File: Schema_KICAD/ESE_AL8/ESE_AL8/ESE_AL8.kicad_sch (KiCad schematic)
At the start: 4 parts

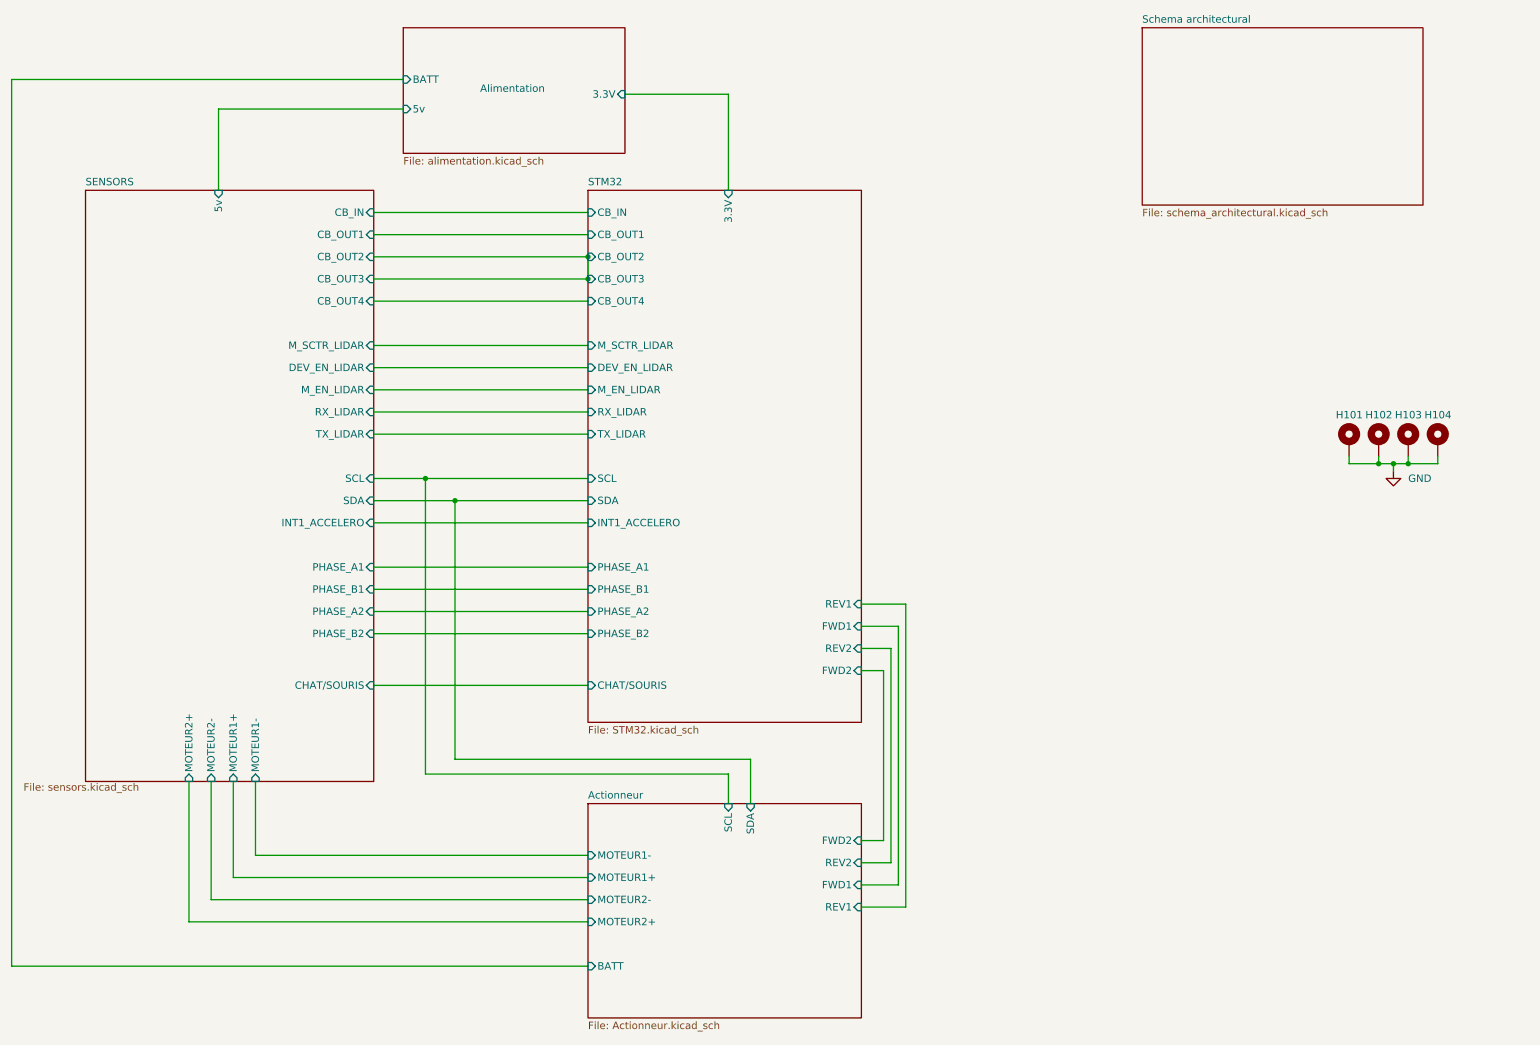
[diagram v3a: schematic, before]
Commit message: commit pour le schema avec 2 CB
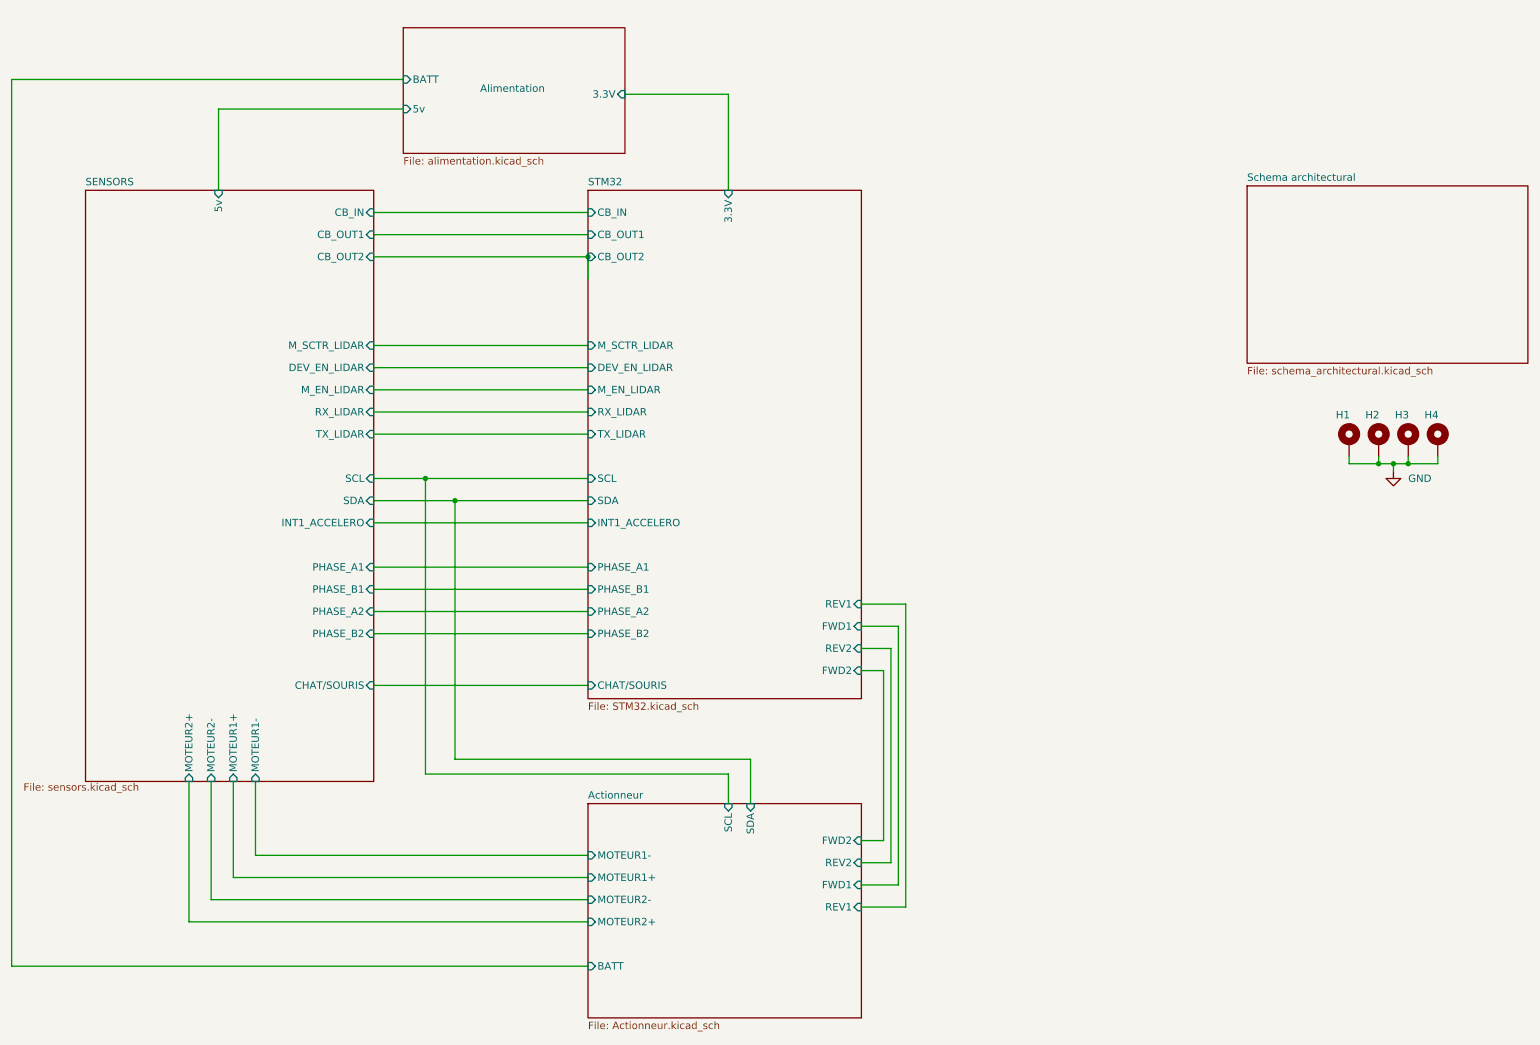
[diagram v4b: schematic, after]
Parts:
- renumbered H101 to H1, H102 to H2, H103 to H3, H104 to H4
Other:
- sheet SENSORS ports: added none; removed CB_OUT3, CB_OUT4
- sheet STM32 ports: added none; removed CB_OUT3, CB_OUT4
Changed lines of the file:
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@@
-	)
-	(junction
-		(at 120.65 64.77)
-		(diameter 0)
-		(color 0 0 0 0)
 	)
 	(junction
@@
 	(wire
 		(pts
-			(xy 83.82 64.77) (xy 120.65 64.77)
-		)
-		(stroke
-			(width 0)
-			(type default)
-		)
-	)
-	(wire
-		(pts
 			(xy 88.9 35.56) (xy 57.15 35.56)
 		)
@@
 		(pts
 			(xy 148.59 147.32) (xy 97.79 147.32)
-		)
-		(stroke
-			(width 0)
-			(type default)
-		)
-	)
-	(wire
-		(pts
-			(xy 83.82 68.58) (xy 120.65 68.58)
 		)
 		(stroke
@@
 		(on_board yes)
 		(dnp no)
-		(property "Reference" "H104"
+		(property "Reference" "H4"
 			(at 264.414 88.138 0)
 			(effects
@@
 			(project "ESE_AL8"
 				(path "/c3d0eb52-cd9d-4e69-bcf7-3f0716f715c6"
-					(reference "H104")
+					(reference "H4")
 					(unit 1)
 				)
@@
 		(on_board yes)
 		(dnp no)
-		(property "Reference" "H103"
+		(property "Reference" "H3"
 			(at 259.334 88.138 0)
 			(effects
@@
 			(project "ESE_AL8"
 				(path "/c3d0eb52-cd9d-4e69-bcf7-3f0716f715c6"
-					(reference "H103")
+					(reference "H3")
 					(unit 1)
 				)
@@
 		(on_board yes)
 		(dnp no)
-		(property "Reference" "H101"
+		(property "Reference" "H1"
 			(at 249.174 88.138 0)
 			(effects
@@
 			(project ""
 				(path "/c3d0eb52-cd9d-4e69-bcf7-3f0716f715c6"
-					(reference "H101")
+					(reference "H1")
 					(unit 1)
 				)
@@
 		(dnp no)
 		(fields_autoplaced yes)
-		(property "Reference" "#PWR0114"
+		(property "Reference" "#PWR01"
 			(at 259.08 104.14 0)
 			(effects
@@
 			(project "ESE_AL8"
 				(path "/c3d0eb52-cd9d-4e69-bcf7-3f0716f715c6"
-					(reference "#PWR0114")
+					(reference "#PWR01")
 					(unit 1)
 				)
@@
 		(on_board yes)
 		(dnp no)
-		(property "Reference" "H102"
+		(property "Reference" "H2"
 			(at 254.254 88.138 0)
 			(effects
@@
 			(project "ESE_AL8"
 				(path "/c3d0eb52-cd9d-4e69-bcf7-3f0716f715c6"
-					(reference "H102")
+					(reference "H2")
 					(unit 1)
 				)
@@
 	(sheet
 		(at 120.65 49.53)
-		(size 46.99 91.44)
+		(size 46.99 87.376)
 		(fields_autoplaced yes)
 		(stroke
@@
 		)
 		(property "Sheetfile" "STM32.kicad_sch"
-			(at 120.65 141.5546 0)
+			(at 120.65 137.4906 0)
 			(effects
 				(font
@@
 		(pin "DEV_EN_LIDAR" input
 			(at 120.65 80.01 180)
-			(effects
-				(font
-					(size 1.27 1.27)
-				)
-				(justify left)
-			)
-		)
-		(pin "CB_OUT4" input
-			(at 120.65 68.58 180)
-			(effects
-				(font
-					(size 1.27 1.27)
-				)
-				(justify left)
-			)
-		)
-		(pin "CB_OUT3" input
-			(at 120.65 64.77 180)
 			(effects
 				(font
@@
 	)
 	(sheet
-		(at 215.9 21.59)
+		(at 233.934 48.768)
 		(size 48.26 30.48)
 		(fields_autoplaced yes)
@@
 		)
 		(property "Sheetname" "Schema architectural"
-			(at 215.9 20.8784 0)
+			(at 233.934 48.0564 0)
 			(effects
 				(font
@@
 		)
 		(property "Sheetfile" "schema_architectural.kicad_sch"
-			(at 215.9 52.6546 0)
+			(at 233.934 79.8326 0)
 			(effects
 				(font
@@
 			(effects
 				(font
-					(size 1.27 1.27)
-				)
-				(justify right)
-			)
-		)
-		(pin "CB_OUT4" input
-			(at 83.82 68.58 0)
-			(effects
-				(font
-					(size 1.27 1.27)
-				)
-				(justify right)
-			)
-		)
-		(pin "CB_OUT3" input
-			(at 83.82 64.77 0)
-			(effects
-				(font
